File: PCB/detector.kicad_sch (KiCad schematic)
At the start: 13 parts, among them J6 Audio In, J7 Through, U2 TL072, U3 LM393

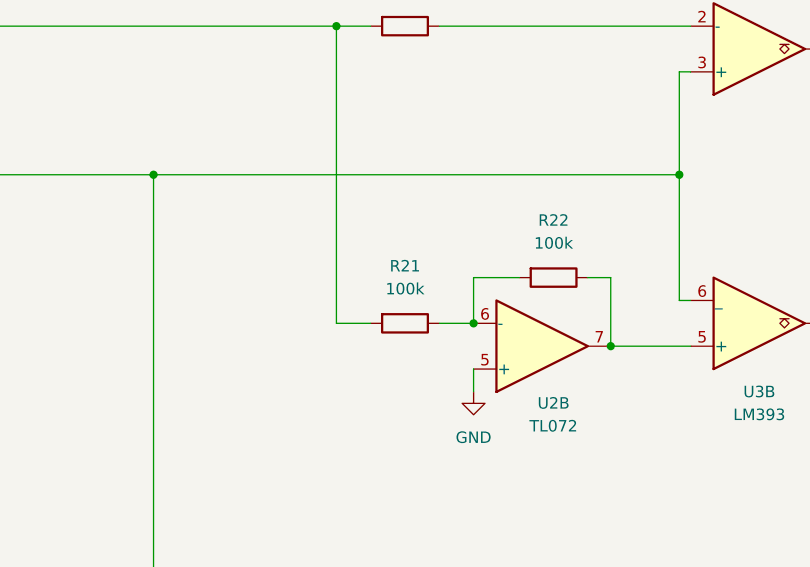
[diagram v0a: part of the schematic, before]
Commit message: PCB layout ready for production
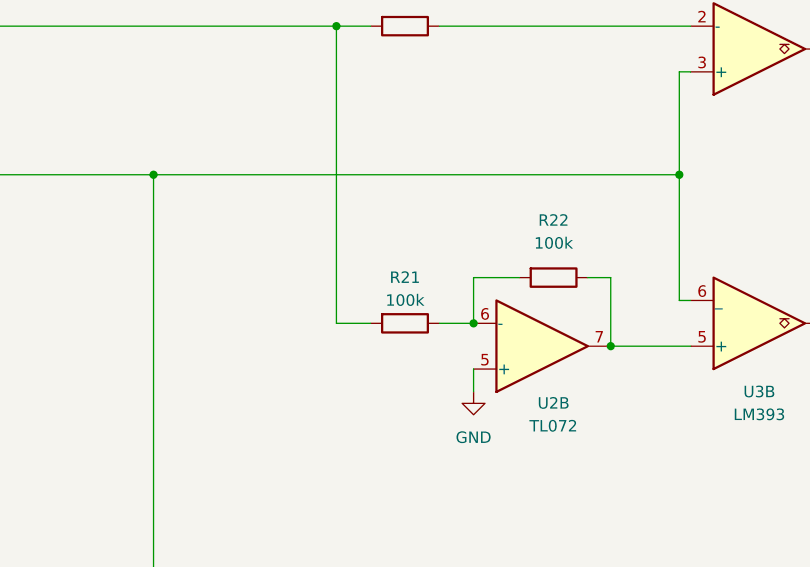
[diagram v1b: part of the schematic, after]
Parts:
- R21: footprint Resistor_THT:R_Axial_DIN0207_L6.3mm_D2.5mm_P7.62mm_Horizontal -> R_Axial_DIN0207_L6.3mm_D2.5mm_P2.54mm_Vertical
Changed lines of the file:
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@@
   (symbol (lib_id "Device:R") (at 151.13 85.09 270) (unit 1)
     (in_bom yes) (on_board yes) (dnp no) (fields_autoplaced)
-    (property "Reference" "R21" (at 151.13 78.74 90)
+    (property "Reference" "R21" (at 151.13 80.01 90)
       (effects (font (size 1.27 1.27)))
     )
-    (property "Value" "100k" (at 151.13 81.28 90)
+    (property "Value" "100k" (at 151.13 82.55 90)
       (effects (font (size 1.27 1.27)))
     )
-    (property "Footprint" "Resistor_THT:R_Axial_DIN0207_L6.3mm_D2.5mm_P7.62mm_Horizontal" (at 151.13 83.312 90)
+    (property "Footprint" "R_Axial_DIN0207_L6.3mm_D2.5mm_P2.54mm_Vertical" (at 151.13 83.312 90)
       (effects (font (size 1.27 1.27)) hide)
     )
